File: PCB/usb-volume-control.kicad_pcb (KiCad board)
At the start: 2 copper layers, 55.9 x 57.8 mm, 17 parts, among them P201 ROT ENC

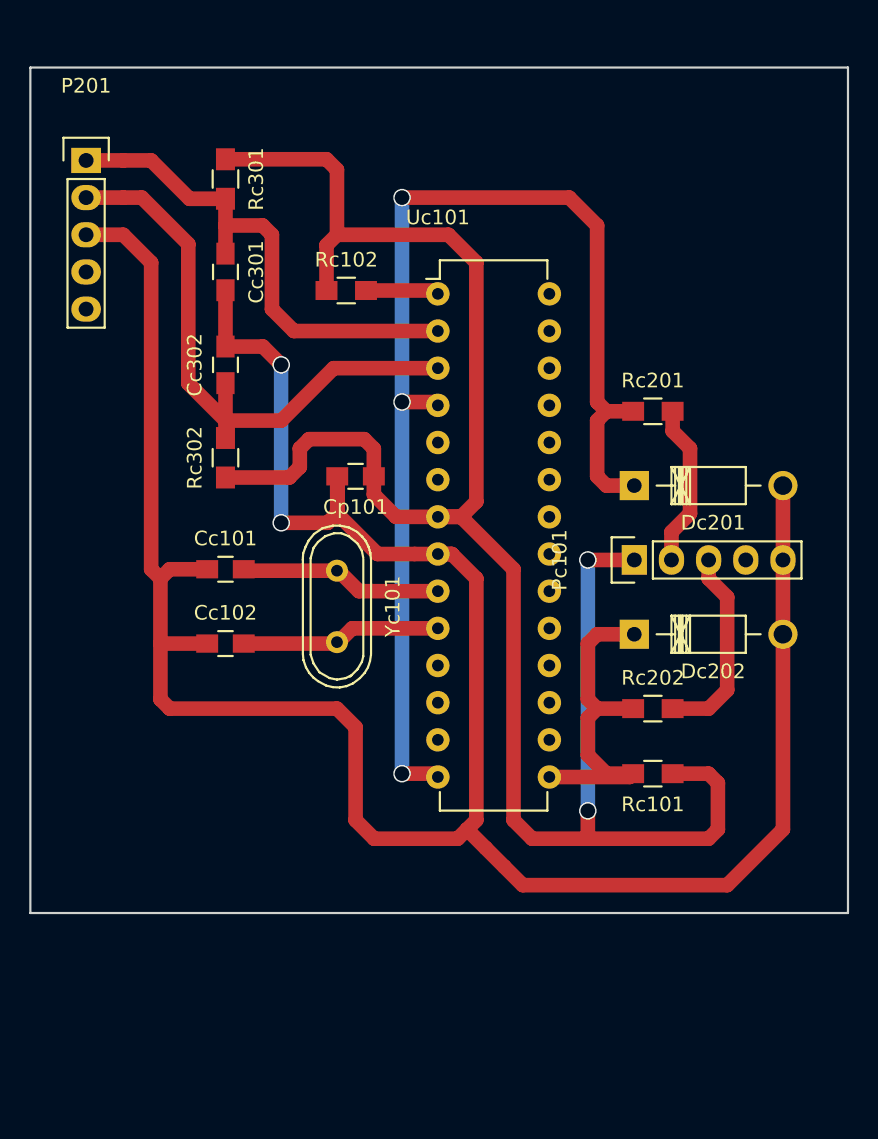
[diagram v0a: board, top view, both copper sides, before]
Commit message: Improved PCB layout
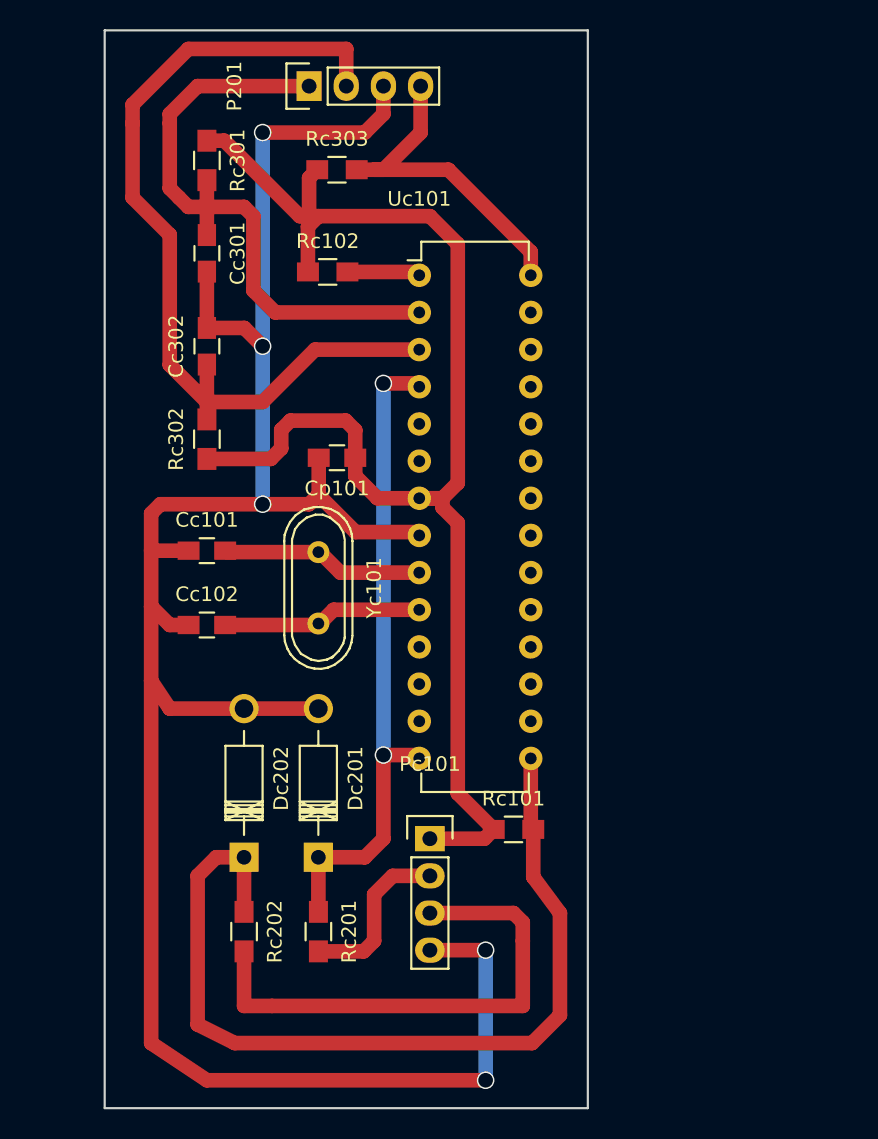
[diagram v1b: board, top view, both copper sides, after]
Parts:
- added Rc303: 2k, Resistors_SMD:R_0805_HandSoldering, F.Cu at (141.6, 96.5)
- P201, Pc101: footprint Pin_Headers:Pin_Header_Straight_1x05 -> Pin_Headers:Pin_Header_Straight_1x04
- moved Rc201 42.3 mm to (140.3, 148.6), turned to 270 degrees
- moved Dc201 33.3 mm to (140.3, 143.5), turned to 90 degrees
- moved Rc202 31.8 mm to (135.3, 148.6), turned to 270 degrees
- moved Dc202 30.7 mm to (135.3, 143.5), turned to 90 degrees
- moved Pc101 23.6 mm to (148.0, 142.2), turned to 0 degrees
- moved P201 16.1 mm to (139.7, 90.8), turned to 90 degrees
- moved Rc101 10.3 mm to (153.7, 141.6), turned to 0 degrees
- moved Cc302 1.80 mm to (132.7, 108.6)
- moved Rc102 1.80 mm to (141.0, 103.5)
- moved Uc101 1.80 mm to (147.2, 103.7)
- moved Cc101 1.80 mm to (132.7, 122.6)
- moved Cc102 1.80 mm to (132.7, 127.6)
- moved Cc301 1.80 mm to (132.7, 102.2)
- moved Cp101 1.80 mm to (141.6, 116.2)
- moved Rc301 1.80 mm to (132.7, 95.9)
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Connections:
- Pc101 pad 4: Net-(Pc101-Pad4) -> GND
- Uc101 pad 28: Net-(Uc101-Pad28) -> Net-(P201-Pad4)
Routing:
- net Net-(Dc202-Pad1): track 23.5 -> 61.7 mm
- net VCC: track 133.9 -> 97.7 mm, vias 2 -> 0
- net Net-(Dc201-Pad1): track 80.9 -> 44.9 mm, vias 3 -> 2
- net Net-(P201-Pad4): track 0.00 -> 23.2 mm
- net Net-(Pc101-Pad3): track 13.7 -> 35.1 mm
- net Net-(Cc302-Pad1): track 41.2 -> 60.9 mm
- net GND: track 177.0 -> 157.4 mm, vias 2 -> 5
- net Net-(Cc301-Pad1): track 34.8 -> 42.7 mm
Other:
- board size 55.9 x 57.8 mm -> 33 x 73.7 mm
